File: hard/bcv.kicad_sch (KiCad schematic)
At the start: 5 parts

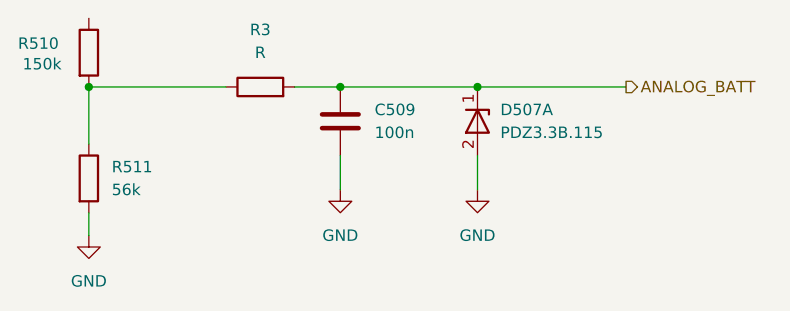
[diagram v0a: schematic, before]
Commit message: edit
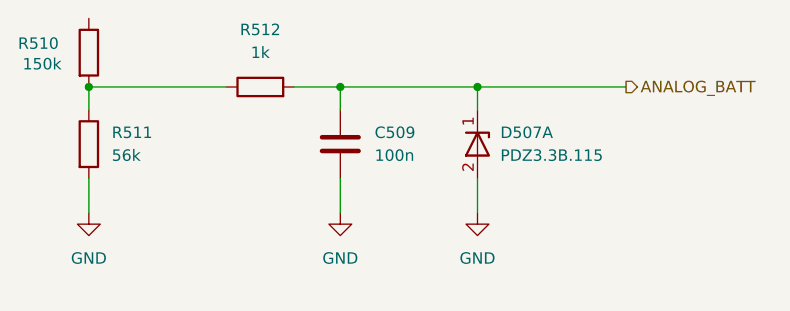
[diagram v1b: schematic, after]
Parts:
- R512: renamed from R3; value R -> 1k
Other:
- moved on the sheet: C509, D507A, R511
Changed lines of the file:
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@@
 	(wire
 		(pts
-			(xy 87.63 86.36) (xy 87.63 82.55)
+			(xy 87.63 88.9) (xy 87.63 85.09)
+		)
+		(stroke
+			(width 0)
+			(type default)
+		)
+	)
+	(wire
+		(pts
+			(xy 102.87 77.47) (xy 102.87 74.93)
 		)
 		(stroke
@@
 	(wire
 		(pts
-			(xy 59.69 74.93) (xy 59.69 81.28)
+			(xy 59.69 74.93) (xy 59.69 77.47)
 		)
 		(stroke
@@
 	(wire
 		(pts
-			(xy 59.69 91.44) (xy 59.69 88.9)
-		)
-		(stroke
-			(width 0)
-			(type default)
-		)
-	)
-	(wire
-		(pts
-			(xy 102.87 82.55) (xy 102.87 86.36)
+			(xy 59.69 88.9) (xy 59.69 85.09)
+		)
+		(stroke
+			(width 0)
+			(type default)
+		)
+	)
+	(wire
+		(pts
+			(xy 87.63 77.47) (xy 87.63 74.93)
+		)
+		(stroke
+			(width 0)
+			(type default)
+		)
+	)
+	(wire
+		(pts
+			(xy 102.87 85.09) (xy 102.87 88.9)
 		)
 		(stroke
@@
 	(symbol
 		(lib_id "power:GND")
-		(at 102.87 86.36 0)
+		(at 102.87 88.9 0)
 		(unit 1)
 		(exclude_from_sim no)
@@
 		(fields_autoplaced yes)
 		(property "Reference" "#PWR06"
-			(at 102.87 92.71 0)
+			(at 102.87 95.25 0)
 			(effects
 				(font
@@
 		)
 		(property "Value" "GND"
-			(at 102.87 91.44 0)
-			(effects
-				(font
-					(size 1.27 1.27)
-				)
-			)
-		)
-		(property "Footprint" ""
-			(at 102.87 86.36 0)
+			(at 102.87 93.98 0)
+			(effects
+				(font
+					(size 1.27 1.27)
+				)
+			)
+		)
+		(property "Footprint" ""
+			(at 102.87 88.9 0)
 			(effects
 				(font
@@
 		)
 		(property "Datasheet" ""
-			(at 102.87 86.36 0)
+			(at 102.87 88.9 0)
 			(effects
 				(font
@@
 		)
 		(property "Description" "Power symbol creates a global label with name \"GND\" , ground"
-			(at 102.87 86.36 0)
+			(at 102.87 88.9 0)
 			(effects
 				(font
@@
 	(symbol
 		(lib_id "Device:C")
-		(at 87.63 78.74 0)
+		(at 87.63 81.28 0)
 		(unit 1)
 		(exclude_from_sim no)
@@
 		(fields_autoplaced yes)
 		(property "Reference" "C509"
-			(at 91.44 77.4699 0)
+			(at 91.44 80.0099 0)
 			(effects
 				(font
@@
 		)
 		(property "Value" "100n"
-			(at 91.44 80.0099 0)
+			(at 91.44 82.5499 0)
 			(effects
 				(font
@@
 		)
 		(property "Footprint" ""
-			(at 88.5952 82.55 0)
+			(at 88.5952 85.09 0)
 			(effects
 				(font
@@
 		)
 		(property "Datasheet" "~"
-			(at 87.63 78.74 0)
+			(at 87.63 81.28 0)
 			(effects
 				(font
@@
 		)
 		(property "Description" "Unpolarized capacitor"
-			(at 87.63 78.74 0)
+			(at 87.63 81.28 0)
 			(effects
 				(font
@@
 	(symbol
 		(lib_id "power:GND")
-		(at 87.63 86.36 0)
+		(at 87.63 88.9 0)
 		(unit 1)
 		(exclude_from_sim no)
@@
 		(fields_autoplaced yes)
 		(property "Reference" "#PWR05"
-			(at 87.63 92.71 0)
+			(at 87.63 95.25 0)
 			(effects
 				(font
@@
 		)
 		(property "Value" "GND"
-			(at 87.63 91.44 0)
-			(effects
-				(font
-					(size 1.27 1.27)
-				)
-			)
-		)
-		(property "Footprint" ""
-			(at 87.63 86.36 0)
+			(at 87.63 93.98 0)
+			(effects
+				(font
+					(size 1.27 1.27)
+				)
+			)
+		)
+		(property "Footprint" ""
+			(at 87.63 88.9 0)
 			(effects
 				(font
@@
 		)
 		(property "Datasheet" ""
-			(at 87.63 86.36 0)
+			(at 87.63 88.9 0)
 			(effects
 				(font
@@
 		)
 		(property "Description" "Power symbol creates a global label with name \"GND\" , ground"
-			(at 87.63 86.36 0)
+			(at 87.63 88.9 0)
 			(effects
 				(font
@@
 	(symbol
 		(lib_id "Device:D_Zener_Dual_CommonAnode_KAK_Split")
-		(at 102.87 78.74 90)
+		(at 102.87 81.28 90)
 		(unit 1)
 		(exclude_from_sim no)
@@
 		(fields_autoplaced yes)
 		(property "Reference" "D507"
-			(at 105.41 77.4699 90)
+			(at 105.41 80.0099 90)
 			(effects
 				(font
@@
 		)
 		(property "Value" "PDZ3.3B.115"
-			(at 105.41 80.0099 90)
+			(at 105.41 82.5499 90)
 			(effects
 				(font
@@
 		)
 		(property "Footprint" ""
-			(at 105.41 81.28 0)
+			(at 105.41 83.82 0)
 			(effects
 				(font
@@
 		)
 		(property "Datasheet" "~"
-			(at 105.41 81.28 0)
+			(at 105.41 83.82 0)
 			(effects
 				(font
@@
 		)
 		(property "Description" "Dual Zener diode, common anode on pin 1"
-			(at 102.87 78.74 0)
+			(at 102.87 81.28 0)
 			(effects
 				(font
@@
 	(symbol
 		(lib_id "power:GND")
-		(at 59.69 91.44 0)
+		(at 59.69 88.9 0)
 		(unit 1)
 		(exclude_from_sim no)
@@
 		(fields_autoplaced yes)
 		(property "Reference" "#PWR04"
-			(at 59.69 97.79 0)
+			(at 59.69 95.25 0)
 			(effects
 				(font
@@
 		)
 		(property "Value" "GND"
-			(at 59.69 96.52 0)
-			(effects
-				(font
-					(size 1.27 1.27)
-				)
-			)
-		)
-		(property "Footprint" ""
-			(at 59.69 91.44 0)
+			(at 59.69 93.98 0)
+			(effects
+				(font
+					(size 1.27 1.27)
+				)
+			)
+		)
+		(property "Footprint" ""
+			(at 59.69 88.9 0)
 			(effects
 				(font
@@
 		)
 		(property "Datasheet" ""
-			(at 59.69 91.44 0)
+			(at 59.69 88.9 0)
 			(effects
 				(font
@@
 		)
 		(property "Description" "Power symbol creates a global label with name \"GND\" , ground"
-			(at 59.69 91.44 0)
+			(at 59.69 88.9 0)
 			(effects
 				(font
@@
 	(symbol
 		(lib_id "Device:R")
-		(at 59.69 85.09 0)
+		(at 59.69 81.28 0)
 		(unit 1)
 		(exclude_from_sim no)
@@
 		(fields_autoplaced yes)
 		(property "Reference" "R511"
-			(at 62.23 83.8199 0)
+			(at 62.23 80.0099 0)
 			(effects
 				(font
@@
 		)
 		(property "Value" "56k"
-			(at 62.23 86.3599 0)
+			(at 62.23 82.5499 0)
 			(effects
 				(font
@@
 		)
 		(property "Footprint" ""
-			(at 57.912 85.09 90)
+			(at 57.912 81.28 90)
 			(effects
 				(font
@@
 		)
 		(property "Datasheet" "~"
-			(at 59.69 85.09 0)
+			(at 59.69 81.28 0)
 			(effects
 				(font
@@
 		)
 		(property "Description" "Resistor"
-			(at 59.69 85.09 0)
+			(at 59.69 81.28 0)
 			(effects
 				(font
@@
 		(dnp no)
 		(fields_autoplaced yes)
-		(property "Reference" "R3"
+		(property "Reference" "R512"
 			(at 78.74 68.58 90)
 			(effects
@@
 			)
 		)
-		(property "Value" "R"
+		(property "Value" "1k"
 			(at 78.74 71.12 90)
 			(effects
@@
 			(project ""
 				(path "/13844229-b559-4868-a710-53f590233cb2/ca9a428d-b29f-459a-8b79-10121d41243b/7ce177ed-6650-4628-99b0-bf88d1bff3a8"
-					(reference "R3")
-					(unit 1)
-				)
+					(reference "R512")
+					(unit 1)
+				)
